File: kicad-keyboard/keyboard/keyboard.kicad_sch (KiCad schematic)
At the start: 85 parts, among them SW1 SW_Push, SW10 SW_Push, SW11 SW_Push, SW12 SW_Push, SW13 SW_Push, SW14 SW_Push, SW15 SW_Push, SW16 SW_Push, SW17 SW_Push, SW18 SW_Push, SW19 SW_Push, SW2 SW_Push, SW20 SW_Push, SW21 SW_Push, SW22 SW_Push, SW23 SW_Push, SW24 SW_Push, SW25 SW_Push, SW26 SW_Push, SW27 SW_Push, SW28 SW_Push, SW29 SW_Push, SW3 SW_Push, SW30 SW_Push, SW31 SW_Push, SW32 SW_Push, SW33 SW_Push, SW34 SW_Push, SW35 SW_Push, SW36 SW_Push, SW37 SW_Push, SW38 SW_Push, SW39 SW_Slide_DPDT, SW4 SW_Push, SW5 SW_Push, SW6 SW_Push, SW7 SW_Push, SW8 SW_Push, SW9 SW_Push, U2 MCP23017_SO

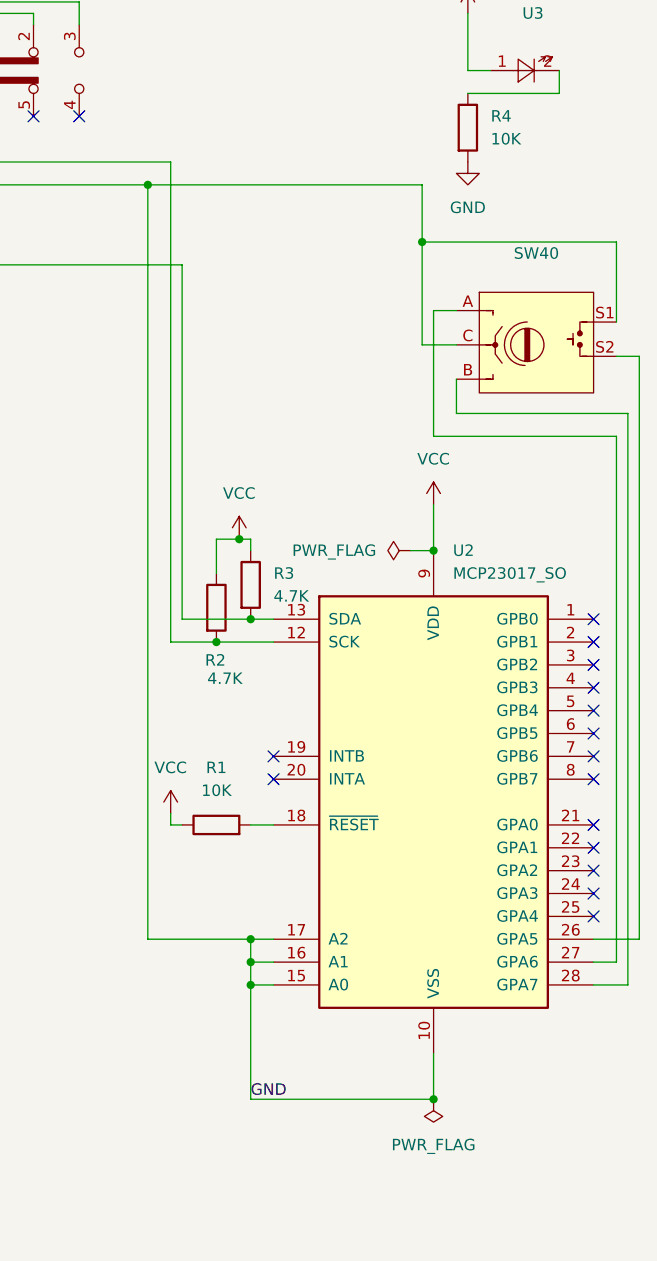
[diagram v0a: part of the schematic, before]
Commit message: add: fix some i2c thing
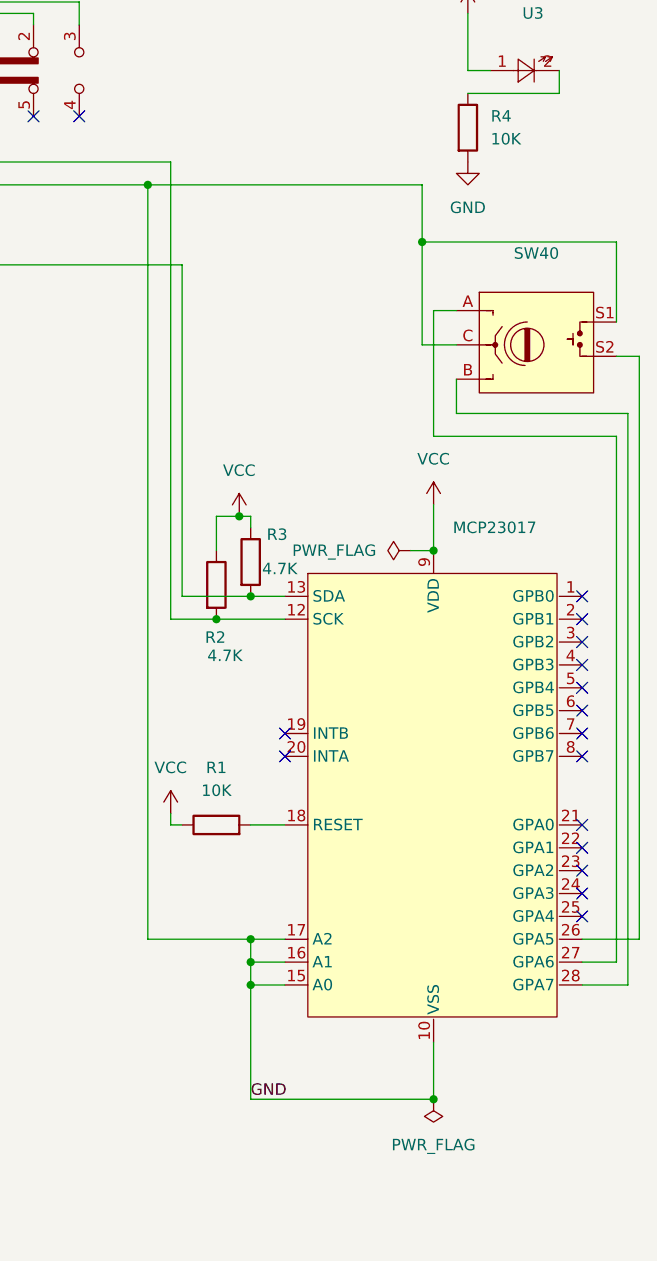
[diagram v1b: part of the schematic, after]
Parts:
- removed U2: MCP23017_SO, Package_SO:SOIC-28W_7.5x17.9mm_P1.27mm, symbol Interface_Expansion:MCP23017_SO
- added MCP23017: ~, Lilyspad:MCP23017, symbol Lilyspad:i2c_expander
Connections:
- net GND: now also MCP23017.10 (VSS), MCP23017.15 (A0), MCP23017.16 (A1), MCP23017.17 (A2)
- net VCC: now also MCP23017.9 (VDD)
- net at R1.2: now also MCP23017.18 (RESET)
- net at R3.2, U1.20 (SDA): now also MCP23017.13 (SDA)
- net at R2.2, U1.21 (SCL): now also MCP23017.12 (SCK)
- net at SW40.S2: now also MCP23017.26 (GPA5)
- net at SW40.A: now also MCP23017.27 (GPA6)
- net at SW40.B: now also MCP23017.28 (GPA7)
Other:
- moved on the sheet: R2, R3
